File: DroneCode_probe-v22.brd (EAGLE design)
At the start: 44 x 22 mm, 67 parts, among them IC1 STM32F103CBT6, IC2 MIC5255-3.3YM5, J1 ARM_MINI_JTAGSMT-S, J2 SM06B-SURS-TF, J3 SH06, J4 JUNCTION, J5 JUNCTION, Q1 NDS332P, U20 NUF2042XV6

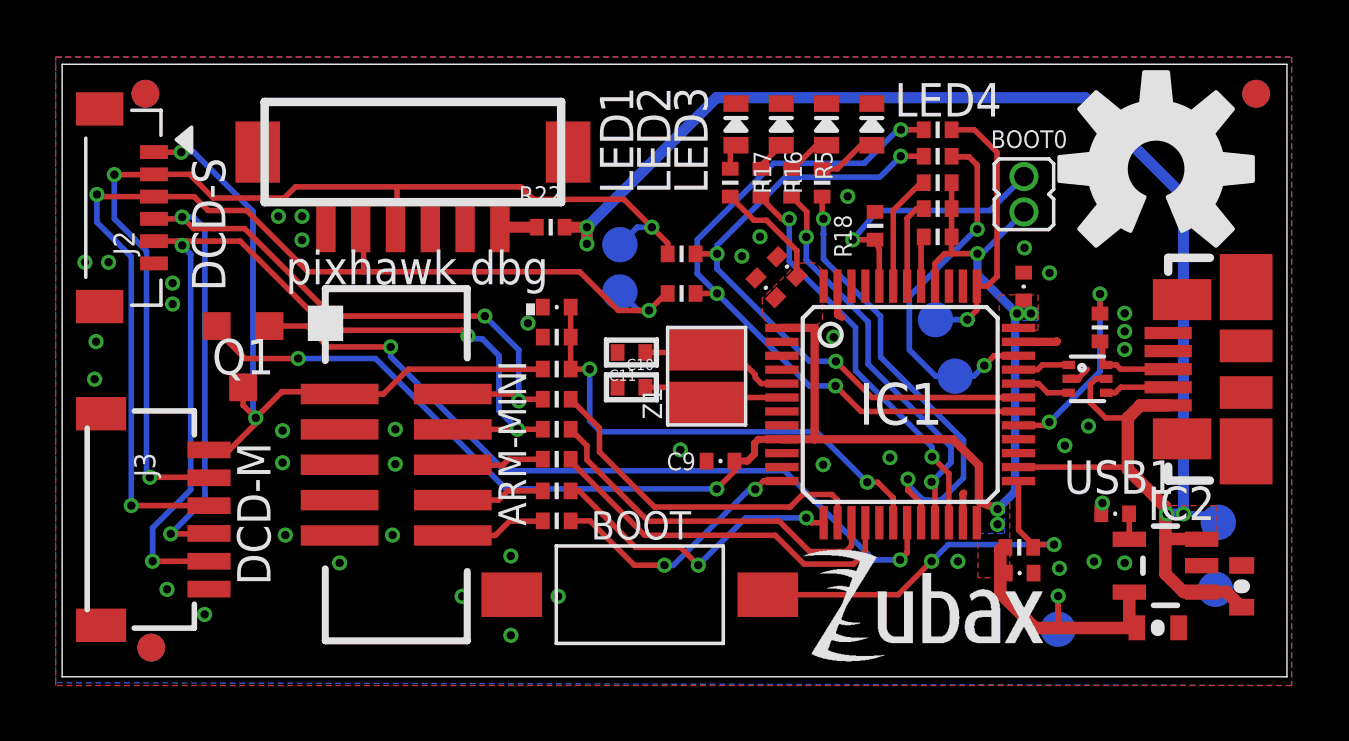
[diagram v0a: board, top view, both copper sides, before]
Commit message: cleanup
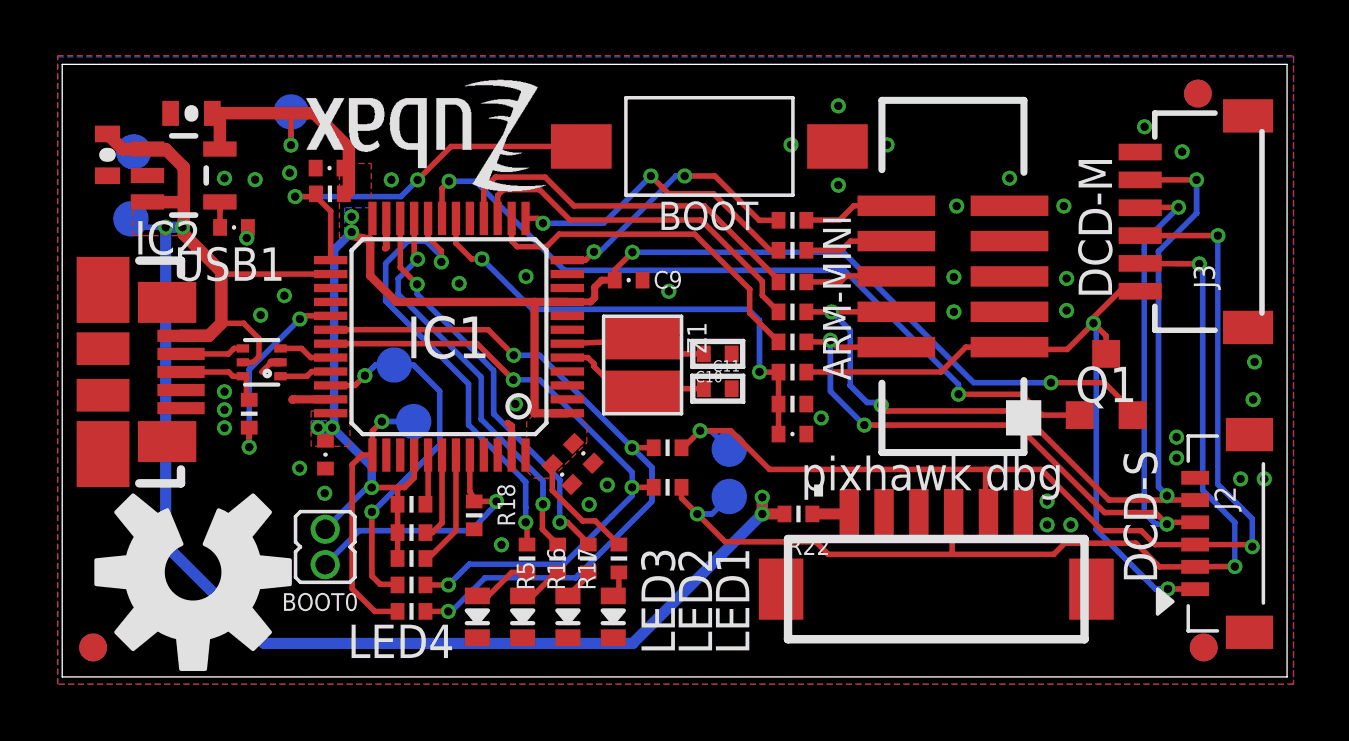
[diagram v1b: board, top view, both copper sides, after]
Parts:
- moved JP1 46.3 mm to (1.11, 1.06), turned to 0 degrees
- moved JP5 46.3 mm to (1.11, 1.06), turned to 180 degrees
- moved J2 44.6 mm to (43.5, 5.15), turned to 90 degrees
- moved C1 43.6 mm to (1.63, 18.8), turned to 270 degrees
- moved J3 43.0 mm to (43.5, 11.9), turned to 90 degrees
- moved JP3 42.9 mm to (41.0, 1.06), turned to 180 degrees
- moved JP6 42.9 mm to (41.0, 1.06), turned to 180 degrees
- moved JP2 42.5 mm to (40.8, 20.9), turned to 0 degrees
- moved JP4 42.5 mm to (40.8, 20.9), turned to 180 degrees
- moved TP4 41.9 mm to (2.57, 18.9), turned to 90 degrees
- moved USB1 41.1 mm to (1.47, 10.9), turned to 0 degrees
- moved TP5 40.6 mm to (2.47, 16.4), turned to 90 degrees
- moved C3 39.3 mm to (4.65, 20.2), turned to 180 degrees
- moved IC2 38.0 mm to (4.37, 18.0), turned to 270 degrees
- moved U$5 37.5 mm to (4.70, 3.76), turned to 180 degrees
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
